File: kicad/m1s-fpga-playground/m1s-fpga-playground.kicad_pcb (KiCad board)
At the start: 4 copper layers, 90 x 65 mm, 188 parts, among them J1 Conn_02x20_Odd_Even, J102 Pin Header, J2 Conn_02x07_Odd_Even, J301 ICD15S13E4GX00LF, J302 CUI_SJ1-3533NG, J501 10029449-101RLF, J702 CUI PJ102, J703 5.08mm, Q501 2N7002, Q502 2N7002, Q503 2N7002, Q701 PMT21EN, SW101 KMR2, SW102 KMR2, SW103 KMR2, SW104 KMR2, SW105 KMR2, U101 W25Q16JLSSIG, U102 ICE40HX4K-TQ144, U103 TLV71312PDBV, U106 AS4C32M8SA, U301 OPA1602, U601 FT2232HL, U603 93LCxxC, U701 AP6503, X101 ECS-2520MV-xxx-xx, Y601 ABM3B-12

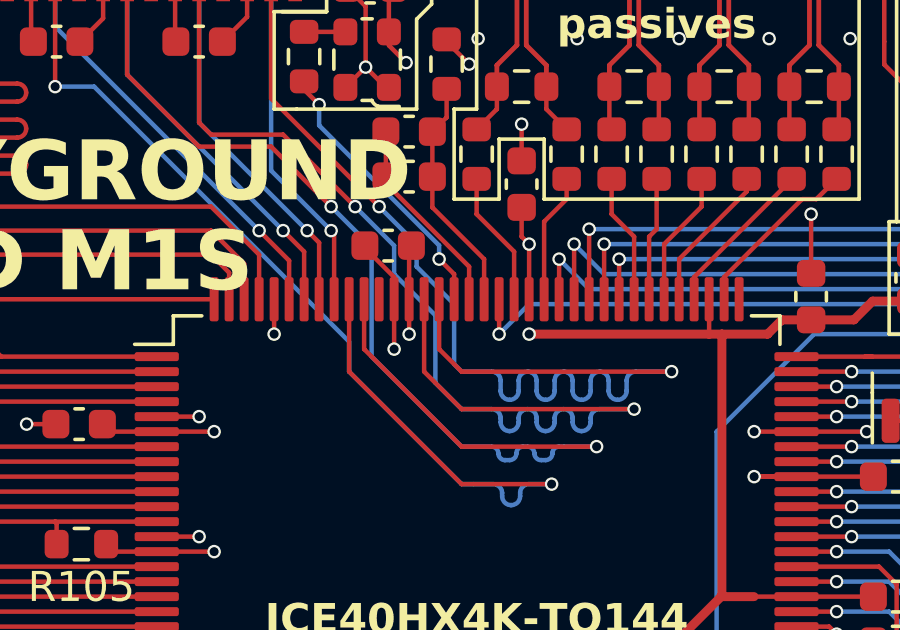
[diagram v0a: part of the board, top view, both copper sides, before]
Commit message: Swapped pins 128 and 129 - PLL conflict
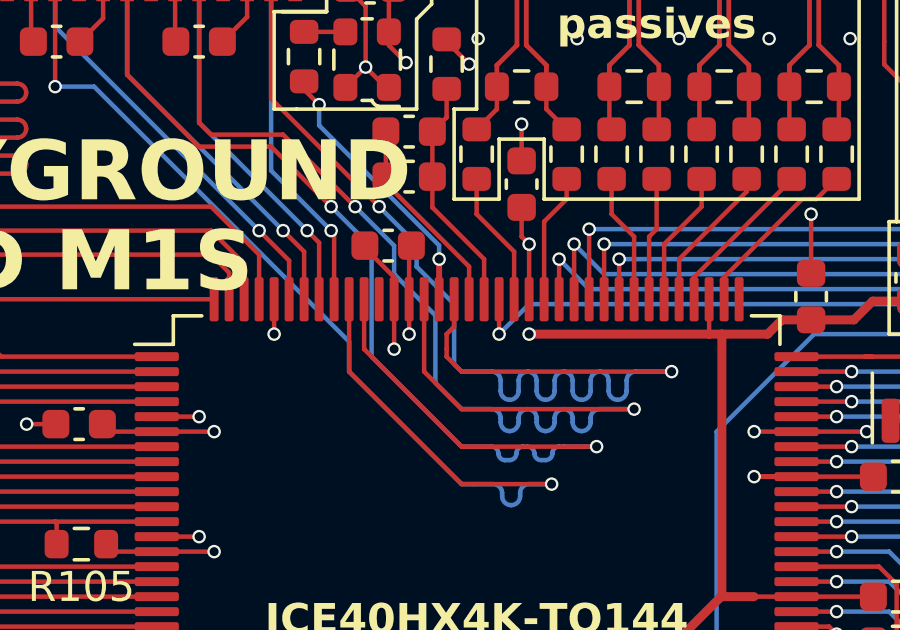
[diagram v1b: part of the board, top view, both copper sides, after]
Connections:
- R101 pad 1: /128 -> /129
- U106 pad 53: /129 -> /128
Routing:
- net /129: track 37.7 -> 9.17 mm
- net /128: track 9.37 -> 37.7 mm
